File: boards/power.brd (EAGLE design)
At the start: 30 x 40 mm, 18 parts, among them IC1 FT232RLSSOP, U1 MAX1555

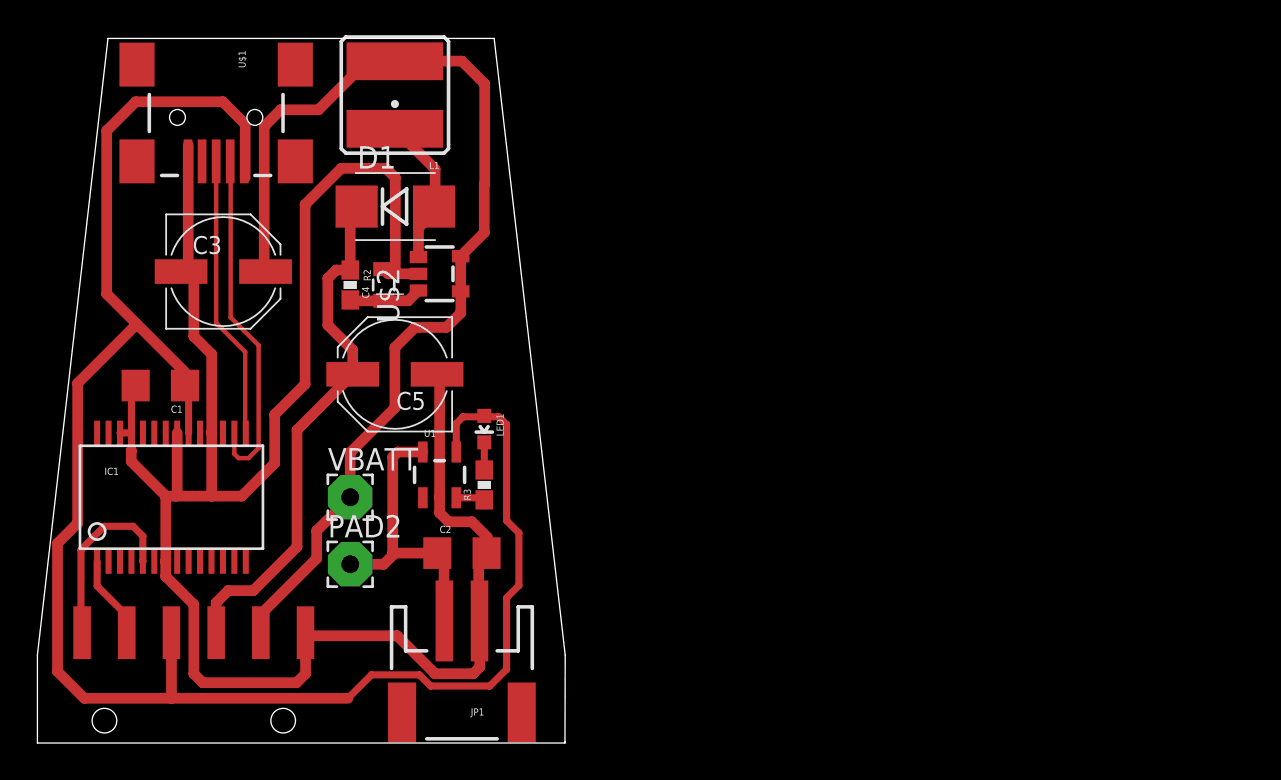
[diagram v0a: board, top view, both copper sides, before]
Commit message: put all the downloaded files into directories
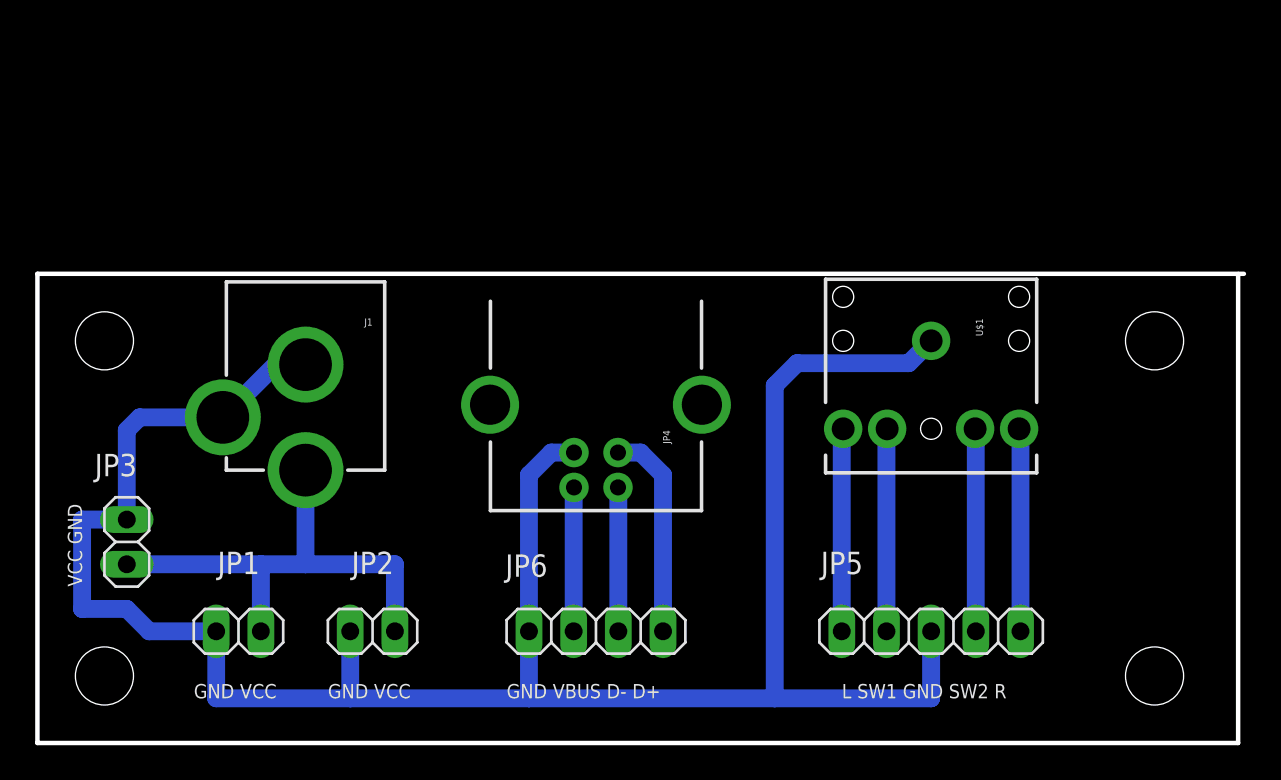
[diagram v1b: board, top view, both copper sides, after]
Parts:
- removed C1, C2: 4.7uF, SparkFun:1206
- removed C3, C5: 100uF, rcl:PANASONIC_D
- removed C4: 1uF, SparkFun:0805
- removed D1: ZHCS2000, SparkFun:SMB-DIODE
- removed IC1: FT232RLSSOP, SparkFun:SSOP28DB
- removed L1: 10uH, SparkFun:CR54
- removed LED1: (no value), SparkFun:LED-0603
- removed PAD2, VBATT: (no value), wirepad:2,54/1,0
- removed R2: 10, SparkFun:0603-RES
- removed R3: 150, SparkFun:0603-RES
- removed U$2: SP6641SP6641A/B, Sipex Custom:SOT23-5
- removed U1: MAX1555, SparkFun:SOT23-5
- added FRAME1: FRAME-LETTER, SparkFun-Aesthetics:CREATIVE_COMMONS
- added J1: POWER_JACKPTH, SparkFun-Connectors:POWER_JACK_PTH
- added JP2: PWR_PI, pinhead:1X02
- added JP4: USB-B, SparkFun-Connectors:USB-B-PTH
- added JP5: AUDIO, pinhead:1X05
- added JP6: USB, pinhead:1X04
- added STANDOFF1, STANDOFF2, STANDOFF3, STANDOFF4: STAND-OFF, SparkFun-Electromechanical:STAND-OFF
- JP1: value Battery -> PWR_AMP; device SparkFun:JST-2-SMD -> pinhead:1X02
- JP3: value (none) -> PWR_LCD; device SparkFun-Connectors:1X06-SMD -> pinhead:1X02
- U$1: value USB-MINIB-5PIN -> AUDIO-JACK2PTH; device SparkFun:USB-MINIB -> SparkFun-Connectors:AUDIO-JACK
- moved U$1 42.6 mm to (50.8, 22.9)
- moved JP1 13.1 mm to (11.4, 6.35)
- moved JP3 10.9 mm to (5.08, 11.4), turned to 90 degrees
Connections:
- removed net D+: IC1.15, U$1.D+
- removed net D-: IC1.16, U$1.D-
- removed net LX: D1.A, L1.P$1, U$2.1
- removed net N$55: C2.1, JP1.2, PAD2.1, U1.5
- removed net RX: IC1.5, JP3.1
- removed net TX: IC1.1, JP3.2
- removed net VBATT: C3.+, JP3.5, L1.P$2, U$2.4, U$2.5, VBATT.1
- removed net VBOOST: C5.+, D1.C, JP3.4, R2.1
- removed net VBUS: C1.1, IC1.20, JP3.3, LED1.A, U$1.VBUS, U1.4
- removed net VCCIO: IC1.4
- removed net VOUT: C4.1, R2.2, U$2.3
- new net N$10: JP4.VBUS, JP6.2
- new net N$11: JP4.D-, JP6.3
- new net N$26: JP5.5, U$1.TIP
- new net N$27: JP5.4, U$1.TSH
- new net N$5: JP5.1, U$1.RING
- new net VCC: J1.PWR, JP1.1, JP2.1, JP3.1
- net GND: now also J1.GND, J1.GNDBREAK, JP1.2, JP2.2, JP3.2, JP4.GND, JP5.3, JP6.1, U$1.SLEEVE; no longer C1.2, C2.2, C3.-, C4.2, C5.-, IC1.18, IC1.21, IC1.25, IC1.26, IC1.7, JP1.1, JP3.6, U$1.GND, U$2.2, U1.2
- net N$2: now also JP4.D+, JP6.4; no longer LED1.C, R3.2
- net N$4: now also JP5.2, U$1.RSH; no longer R3.1, U1.3
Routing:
- net VBUS: track 105.2 -> 0.00 mm
- net VBATT: track 61.6 -> 0.00 mm
- net VBOOST: track 31.2 -> 0.00 mm
- net VCC: track 0.00 -> 26.7 mm
- net D-: track 19.9 -> 0.00 mm
- net N$55: track 16.8 -> 0.00 mm
- net D+: track 16.2 -> 0.00 mm
- net N$5: track 0.00 -> 11.4 mm
- net N$27: track 0.00 -> 11.4 mm
- net N$26: track 0.00 -> 11.4 mm
- net RX: track 10.7 -> 0.00 mm
- net N$2: track 1.57 -> 12.0 mm
- net N$4: track 1.64 -> 11.4 mm
- net LX: track 9.23 -> 0.00 mm
- net N$11: track 0.00 -> 7.62 mm
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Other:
- board size 30 x 40 mm -> 68.6 x 26.7 mm
- board text added: "GND VBUS D- D+"
- board text added: "GND VCC"
- board text added: "L SW1 GND SW2 R"
- board text added: "VCC GND"
